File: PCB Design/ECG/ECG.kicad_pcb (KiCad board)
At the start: 2 copper layers, 41.9 x 48.9 mm, 45 parts, among them J1 01x05_Female, J2 JST_01x04_Male, U1 Li-Po, U10 ESP32-C3-MINI-1-N4, U2 TP4056-C21417, U3 USBLC6-2SC6, U4 Battery_Switch, U5 5V_switch, U6 TLV62568DBV, U7 MCU_switch, U8 Tactile_push_button_6x6mm, U9 USB-TYPE0-C-16P

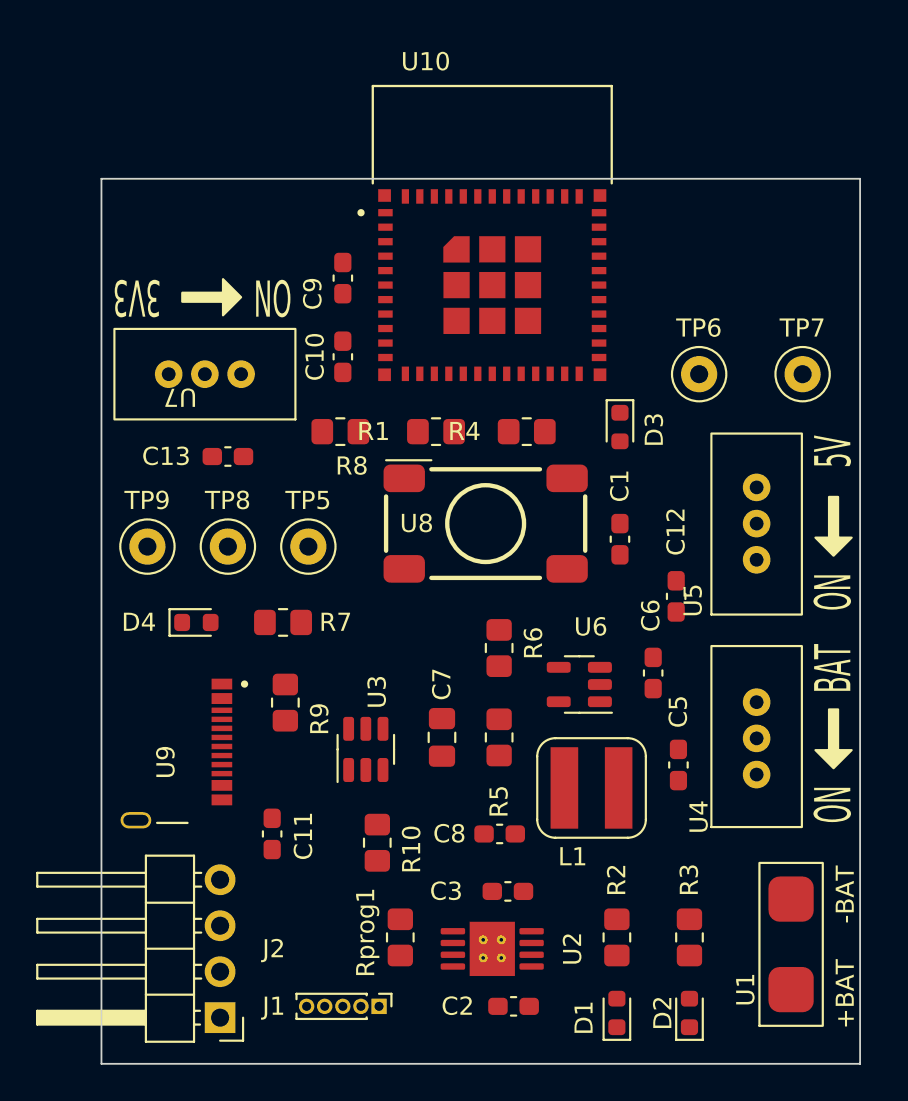
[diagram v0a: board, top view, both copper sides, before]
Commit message: second last iteration hopefully
pcb design, pending Bruno approval
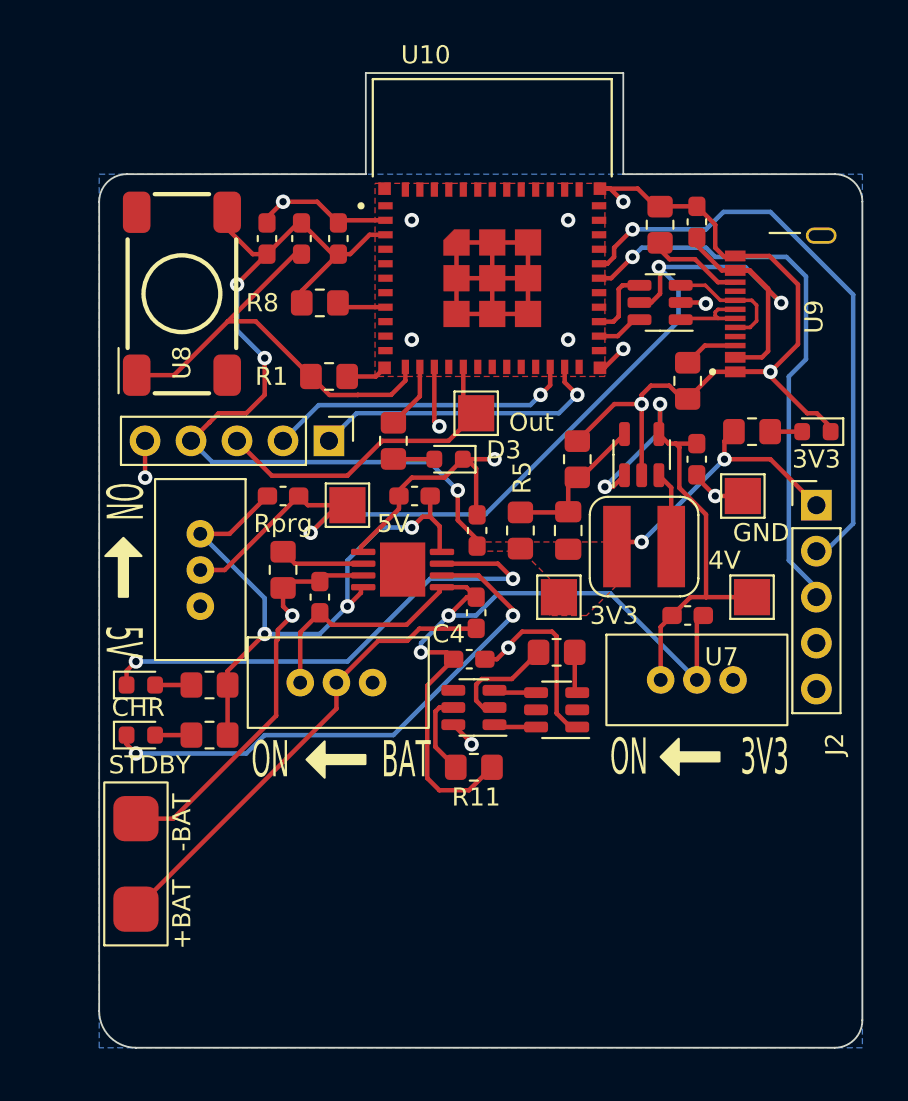
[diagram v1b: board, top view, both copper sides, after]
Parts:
- added C4: 0.1uF, Capacitor_SMD:C_0603_1608Metric_Pad1.08x0.95mm_HandSolder, F.Cu at (234.3, 101.5)
- added R11: 100R, Resistor_SMD:R_0805_2012Metric_Pad1.20x1.40mm_HandSolder, F.Cu at (234.6, 107.4)
- added R12: 1K, Resistor_SMD:R_0805_2012Metric_Pad1.20x1.40mm_HandSolder, F.Cu at (239.1, 101.1)
- added U11: FS8205A, Package_TO_SOT_SMD:SOT-23-6, F.Cu at (239.1, 104.3)
- added U12: DW01, Package_TO_SOT_SMD:SOT-23-6, F.Cu at (234.6, 104.1)
- 3V3: renamed from TP6; footprint TestPoint:TestPoint_Loop_D1.80mm_Drill1.0mm_Beaded -> TestPoint:TestPoint_Pad_2.0x2.0mm
- 4V: renamed from TP9; footprint TestPoint:TestPoint_Loop_D1.80mm_Drill1.0mm_Beaded -> TestPoint:TestPoint_Pad_2.0x2.0mm
- 5V: renamed from TP8; footprint TestPoint:TestPoint_Loop_D1.80mm_Drill1.0mm_Beaded -> TestPoint:TestPoint_Pad_2.0x2.0mm
- GND: renamed from TP7; footprint TestPoint:TestPoint_Loop_D1.80mm_Drill1.0mm_Beaded -> TestPoint:TestPoint_Pad_2.0x2.0mm
- J1: footprint Connector_PinHeader_1.00mm:PinHeader_1x05_P1.00mm_Vertical -> Connector_PinHeader_2.54mm:PinHeader_1x05_P2.54mm_Vertical
- J2: footprint Connector_PinHeader_2.54mm:PinHeader_1x04_P2.54mm_Horizontal -> Connector_PinHeader_2.54mm:PinHeader_1x05_P2.54mm_Vertical
- Out: renamed from TP5; footprint TestPoint:TestPoint_Loop_D1.80mm_Drill1.0mm_Beaded -> TestPoint:TestPoint_Pad_2.0x2.0mm
- R2, R3: value 220 -> 1K
- U2: footprint Package_SO:MSOP-8-1EP_3x3mm_P0.65mm_EP2.5x3mm_Mask1.73x2.36mm_ThermalVias -> Package_SO:MSOP-8-1EP_3x3mm_P0.65mm_EP2.5x3mm_Mask1.73x2.36mm
- moved U9 44.6 mm to (253.8, 82.4), turned to 90 degrees
- moved J2 43.4 mm to (253.5, 93.0), turned to 0 degrees
- moved C11 41.2 mm to (246.9, 77.3), turned to 90 degrees
- moved R10 37.5 mm to (244.9, 77.5), turned to 90 degrees
- moved U1 36.5 mm to (215.9, 113.0)
- moved 3V3 35.8 mm to (253.5, 88.9), turned to 180 degrees
- moved STDBY 34.0 mm to (216.2, 105.7), turned to 0 degrees
- moved 4V 33.5 mm to (249.9, 98.0)
- moved U7 32.0 mm to (246.9, 102.6), turned to 0 degrees
- moved CHR 31.9 mm to (216.2, 102.9), turned to 0 degrees
- moved J1 31.4 mm to (226.6, 89.4)
- moved U5 30.8 mm to (219.5, 96.5), turned to -90 degrees
- moved U3 29.6 mm to (244.9, 81.8), turned to 180 degrees
- moved R3 28.8 mm to (220.0, 105.7), turned to 0 degrees
- moved R9 28.5 mm to (246.4, 86.1), turned to -90 degrees
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- renumbered D4 to 3V3, D1 to CHR, Rprog1 to Rprg, D2 to STDBY
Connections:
- U10 pad 53: (no net) -> GND
- U2 pad 4: In_5V -> +5V
- U3 pad 3: DNO -> DP
- U3 pad 5: unconnected-(U3-Pad5) -> In_5V
- U3 pad 6: DP -> DNO
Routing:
- net GND: track 0.00 -> 138.7 mm, vias 0 -> 17
- net +3V3: track 0.00 -> 66.3 mm, vias 0 -> 5
- net In_5V: track 0.00 -> 65.8 mm, vias 0 -> 3
- net +BATT: track 0.00 -> 52.5 mm, vias 0 -> 2
- net +5V: track 0.00 -> 36.1 mm, vias 0 -> 3
- net /TX: track 0.00 -> 32.2 mm, vias 0 -> 1
- net /RX: track 0.00 -> 31.7 mm, vias 0 -> 1
- net Net-(D2-Pad1): track 0.00 -> 30.4 mm, vias 0 -> 2
- net +4V: track 0.00 -> 29.0 mm, vias 0 -> 2
- net Net-(D1-Pad1): track 0.00 -> 28.6 mm, vias 0 -> 2
- net BatO: track 0.00 -> 26.1 mm
- net BTN: track 0.00 -> 23.9 mm
- net Output: track 0.00 -> 18.3 mm
- net -LO: track 0.00 -> 17.0 mm, vias 0 -> 1
- net +LO: track 0.00 -> 16.6 mm, vias 0 -> 1
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- added copper zone on F.Cu, net +3V3
- added copper zone on B.Cu, net GND
- added copper zone on F.Cu, net GND
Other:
- board size 41.9 x 48.9 mm -> 42.2 x 53.8 mm
